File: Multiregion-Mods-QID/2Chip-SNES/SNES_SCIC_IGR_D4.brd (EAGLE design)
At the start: 88.9 x 37.5 mm, 27 parts, among them IC1 74HC27D, IC2 74HC30D

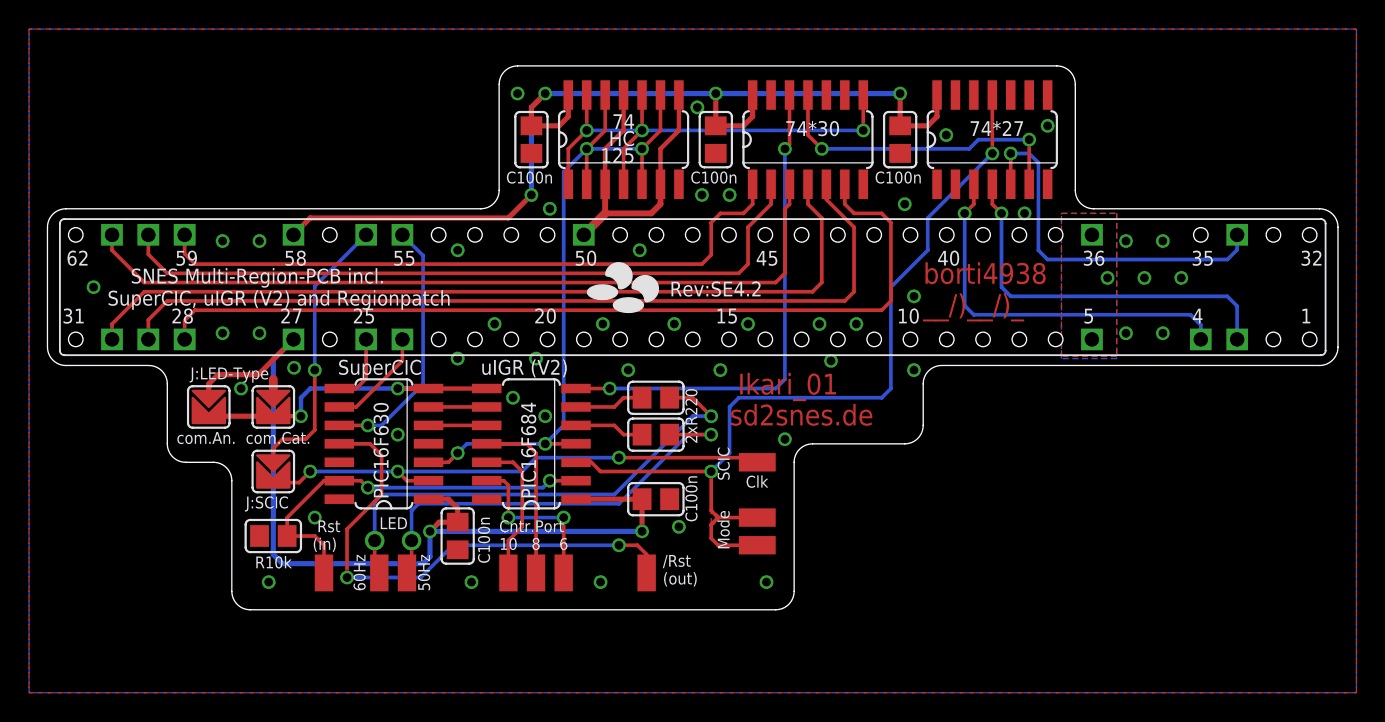
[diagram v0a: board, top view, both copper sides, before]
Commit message: Update Design: - minor changes and adjustments
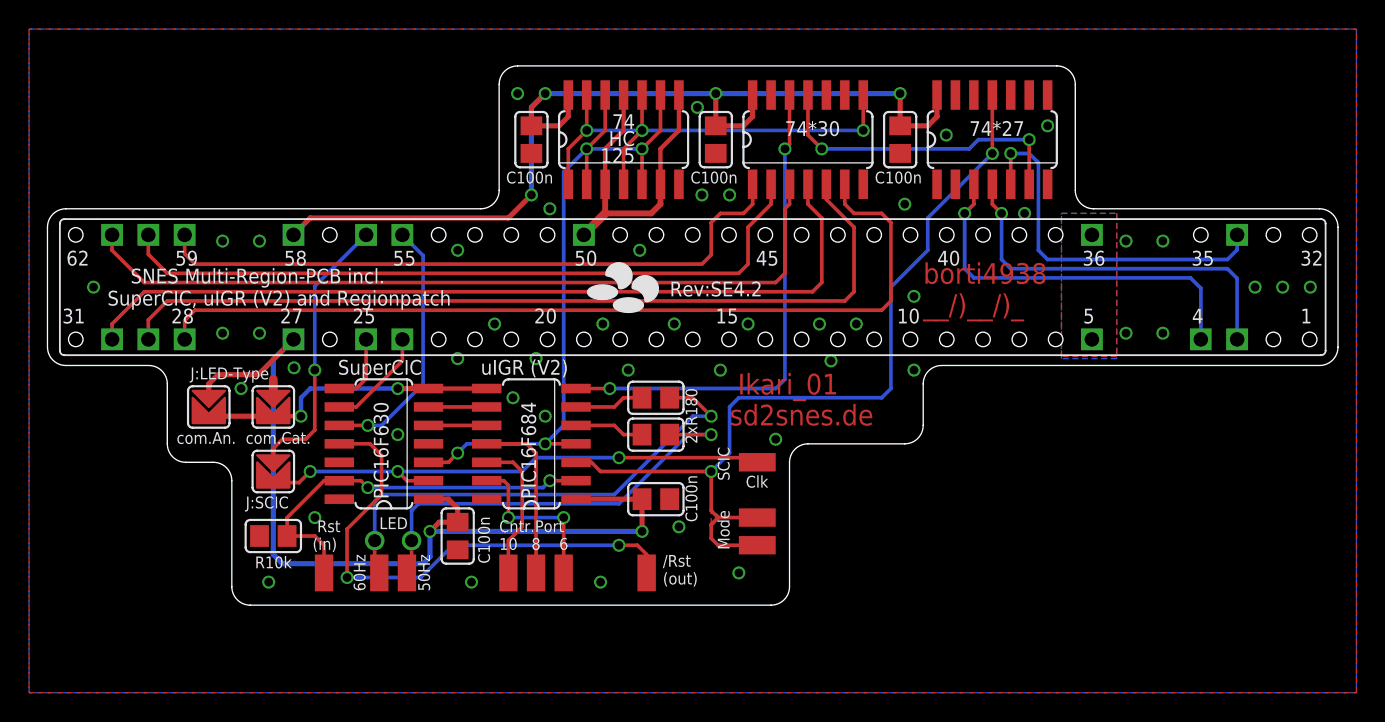
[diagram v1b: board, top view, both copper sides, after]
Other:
- board size 88.9 x 37.5 mm -> 88.9 x 37.1 mm
- board text added: "2xR180"
- board text removed: "2xR220"
